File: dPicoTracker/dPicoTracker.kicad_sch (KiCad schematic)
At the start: 26 parts, among them J1 Conn_01x02_Pin, P1 USB_C_Plug_USB2.0, U1 RP2040, U2 NCP1117-3.3_SOT223, U3 CJ431, U4 CJ431, U5 TPS61221DCK, U6 W25Q128JVS, U7 MAX809STRG, X1 ABM8-272-T3

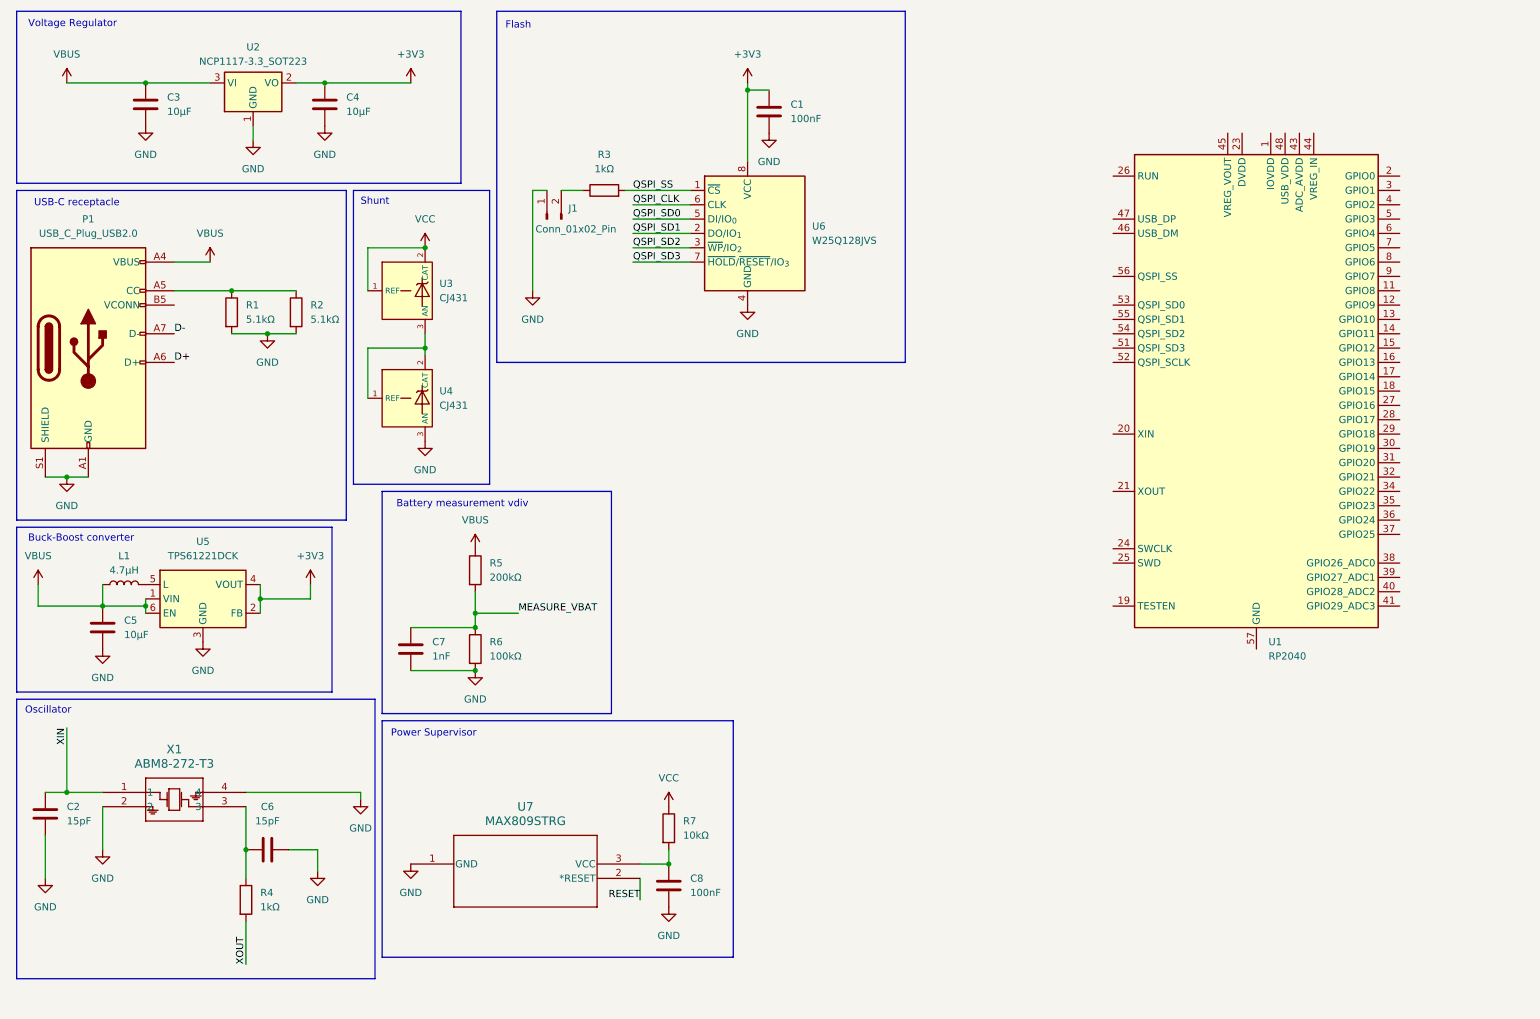
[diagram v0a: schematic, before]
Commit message: add VFO
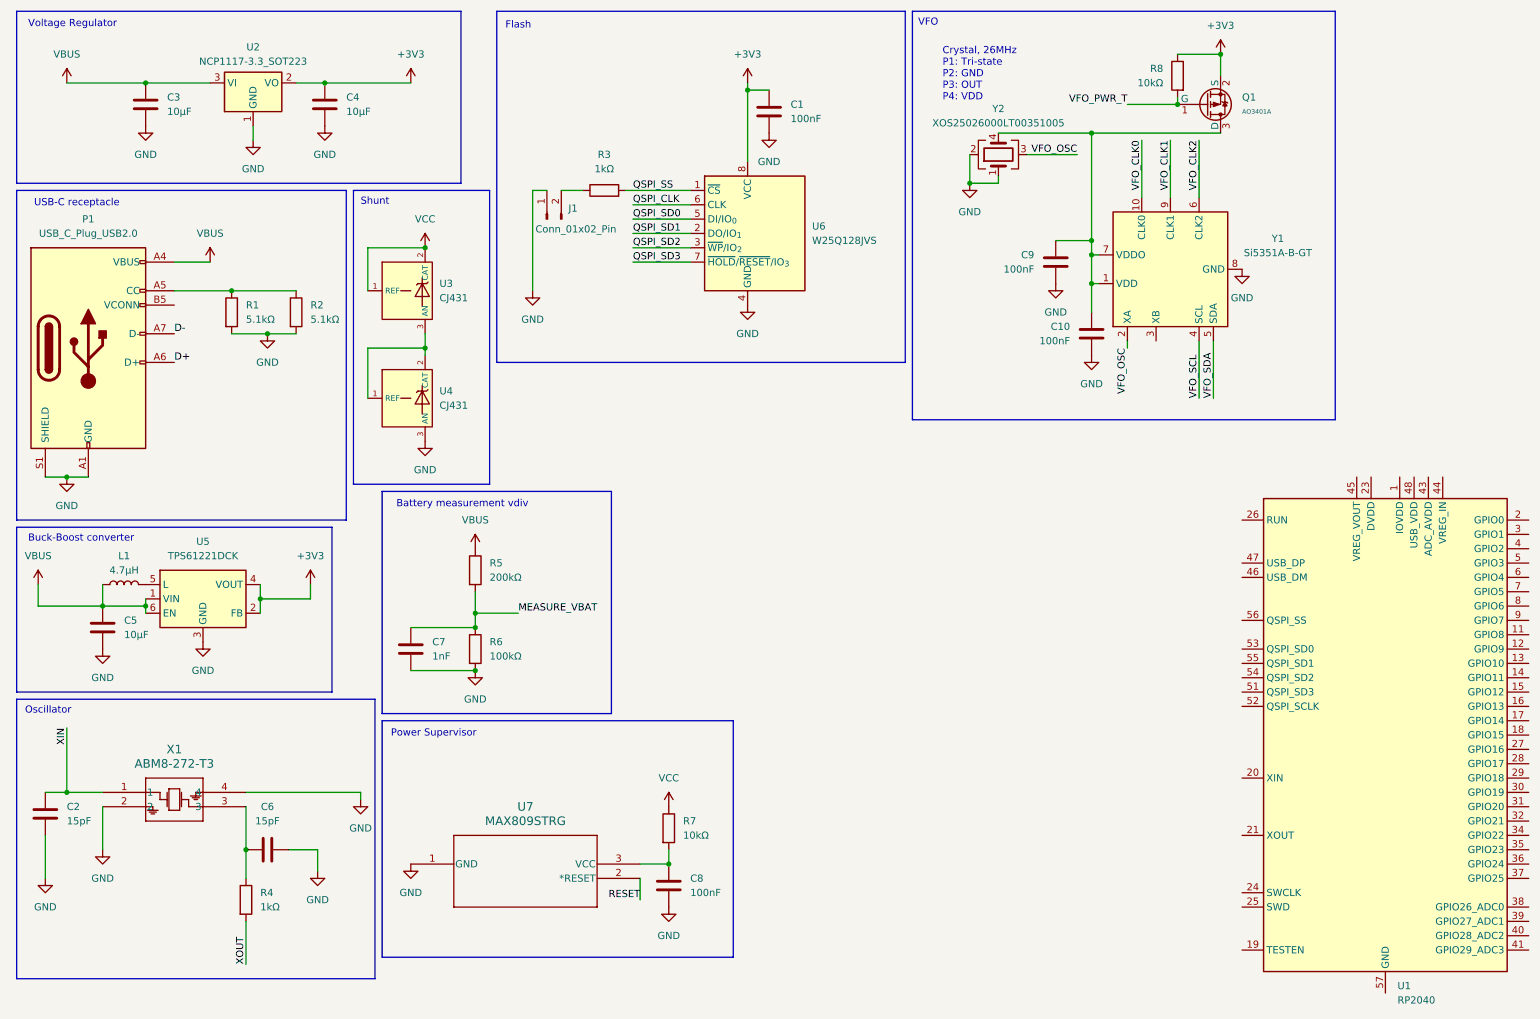
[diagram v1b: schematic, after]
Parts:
- added C10, C9: 100nF, symbol Device:C
- added Q1: AO3401A, PCM_JLCPCB:Q_SOT-23, symbol PCM_JLCPCB-Transistors:PMOS,AO3401A
- added R8: 10kΩ, symbol Device:R
- added Y1: Si5351A-B-GT, Package_SO:MSOP-10_3x3mm_P0.5mm, symbol Oscillator:Si5351A-B-GT
- added Y2: XOS25026000LT00351005, Crystal:Crystal_SMD_2520-4Pin_2.5x2.0mm, symbol Device:Crystal_GND23
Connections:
- net +3V3: now also Q1.2 (S), R8.1
- net GND: now also C10.2, C9.2, Y1.8 (GND), Y2.1, Y2.2
- new net: C10.1, C9.1, Q1.3 (D), Y1.1 (VDD), Y1.7 (VDDO), Y2.4
- new net VFO_CLK0: Y1.10 (CLK0)
- new net VFO_CLK1: Y1.9 (CLK1)
- new net VFO_CLK2: Y1.6 (CLK2)
- new net VFO_OSC: Y1.2 (XA), Y2.3
- new net VFO_PWR_T: Q1.1 (G), R8.2
- new net VFO_SCL: Y1.4 (SCL)
- new net VFO_SDA: Y1.5 (SDA)
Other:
- note added: "Crystal, 26MHz P1: Tri-state P2: GND P3: OUT P4: VDD"
- note added: "VFO"
- moved on the sheet: U1
